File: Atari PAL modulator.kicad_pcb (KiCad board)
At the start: 2 copper layers, 115 x 50 mm, 37 parts, among them J1 Conn_01x08, J2 Conn_01x08, J3 DIN-5_180degree, J4 Conn_01x02, Q1 MMBT3904, Q2 MMBT2222, Q3 MMBT2222, Q4 MMBT3904, U1 4050

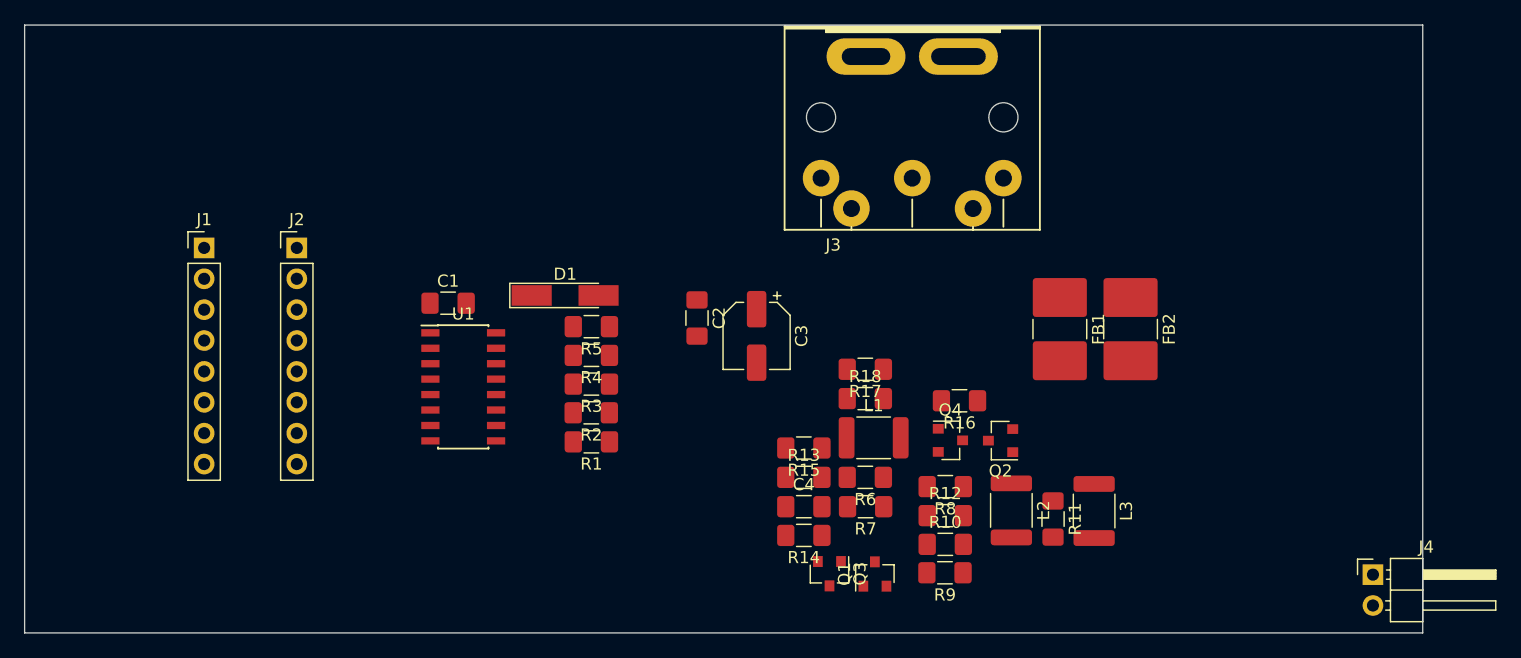
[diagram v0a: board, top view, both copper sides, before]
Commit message: All connections
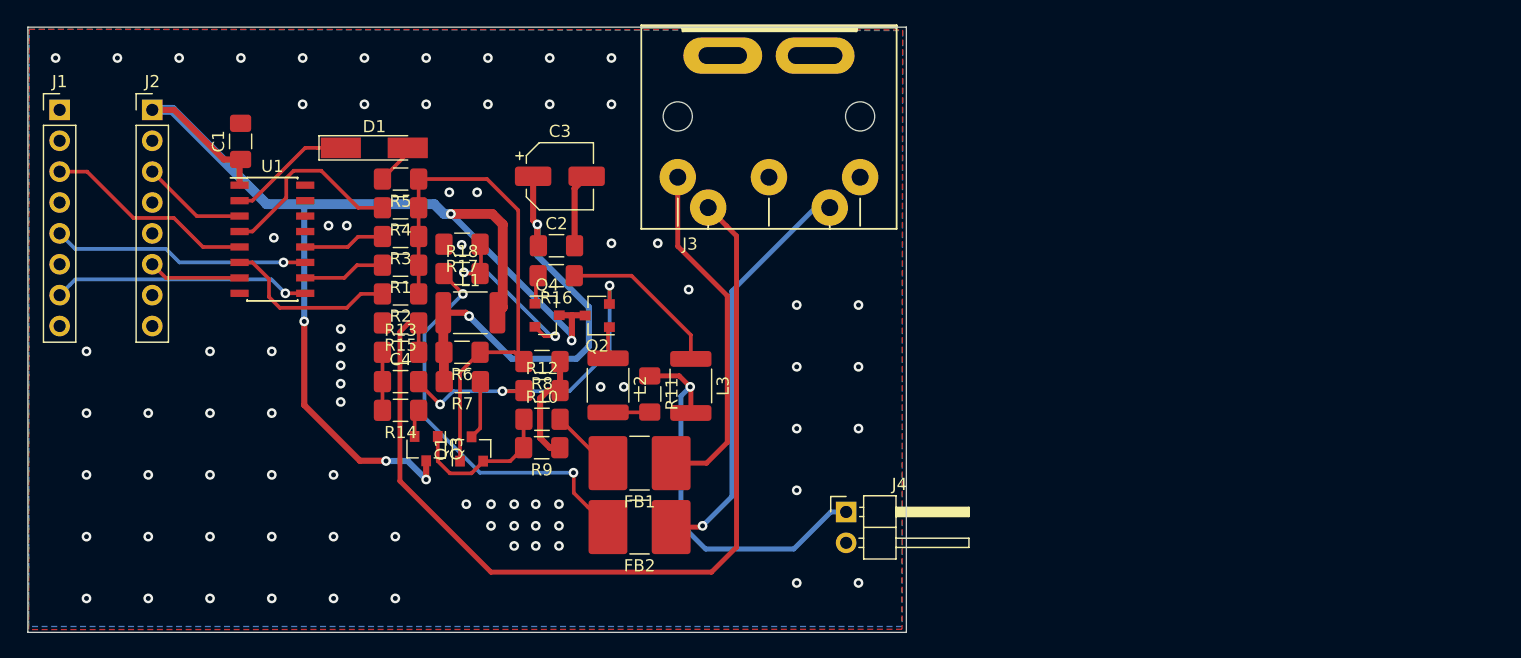
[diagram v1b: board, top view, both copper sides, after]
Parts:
- moved J4 43.6 mm to (147.6, 130.0)
- moved FB2 43.5 mm to (130.6, 131.3), turned to 180 degrees
- moved FB1 36.3 mm to (130.6, 126.0), turned to 180 degrees
- moved L2 34.7 mm to (128.0, 119.6)
- moved L3 34.7 mm to (134.8, 119.7)
- moved Q1 34.7 mm to (116.8, 124.9)
- moved Q3 34.7 mm to (113.0, 124.8)
- moved R11 34.7 mm to (131.4, 120.3)
- moved R16 34.7 mm to (123.7, 110.6)
- moved R7 34.7 mm to (116.0, 119.3)
- moved C4 34.7 mm to (110.9, 119.3)
- moved L1 34.7 mm to (116.7, 113.7)
- moved Q2 34.7 mm to (127.1, 113.9)
- moved Q4 34.7 mm to (123.0, 113.9)
- moved R13 34.7 mm to (110.9, 116.9)
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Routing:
- net VCC: track 0.00 -> 100.8 mm, vias 0 -> 5
- net COMPOSITE: track 0.00 -> 77.1 mm
- net Net-(Q1-Pad1): track 0.00 -> 44.9 mm
- net Net-(C2-Pad1): track 0.00 -> 37.5 mm, vias 0 -> 2
- net COLOR: track 0.00 -> 34.2 mm, vias 0 -> 1
- net CHROMA: track 0.00 -> 33.8 mm, vias 0 -> 1
- net Net-(FB2-Pad2): track 0.00 -> 33.6 mm, vias 0 -> 2
- net MONO: track 0.00 -> 28.8 mm
- net Net-(C4-Pad2): track 0.00 -> 27.1 mm, vias 0 -> 3
- net LUM0: track 0.00 -> 21.2 mm, vias 0 -> 1
- net LUM2: track 0.00 -> 21.2 mm, vias 0 -> 1
- net LUM3: track 0.00 -> 17.4 mm
- net Net-(R4-Pad2): track 0.00 -> 16.0 mm
- net GND: track 0.00 -> 15.6 mm, vias 0 -> 77
- net Net-(Q4-Pad2): track 0.00 -> 15.5 mm, vias 0 -> 2
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- added copper zone on B.Cu, net GND
- added copper zone on F.Cu, net GND
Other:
- board size 115 x 50 mm -> 72.3 x 49.8 mm
